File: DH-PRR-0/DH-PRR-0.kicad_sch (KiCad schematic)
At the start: 0 parts

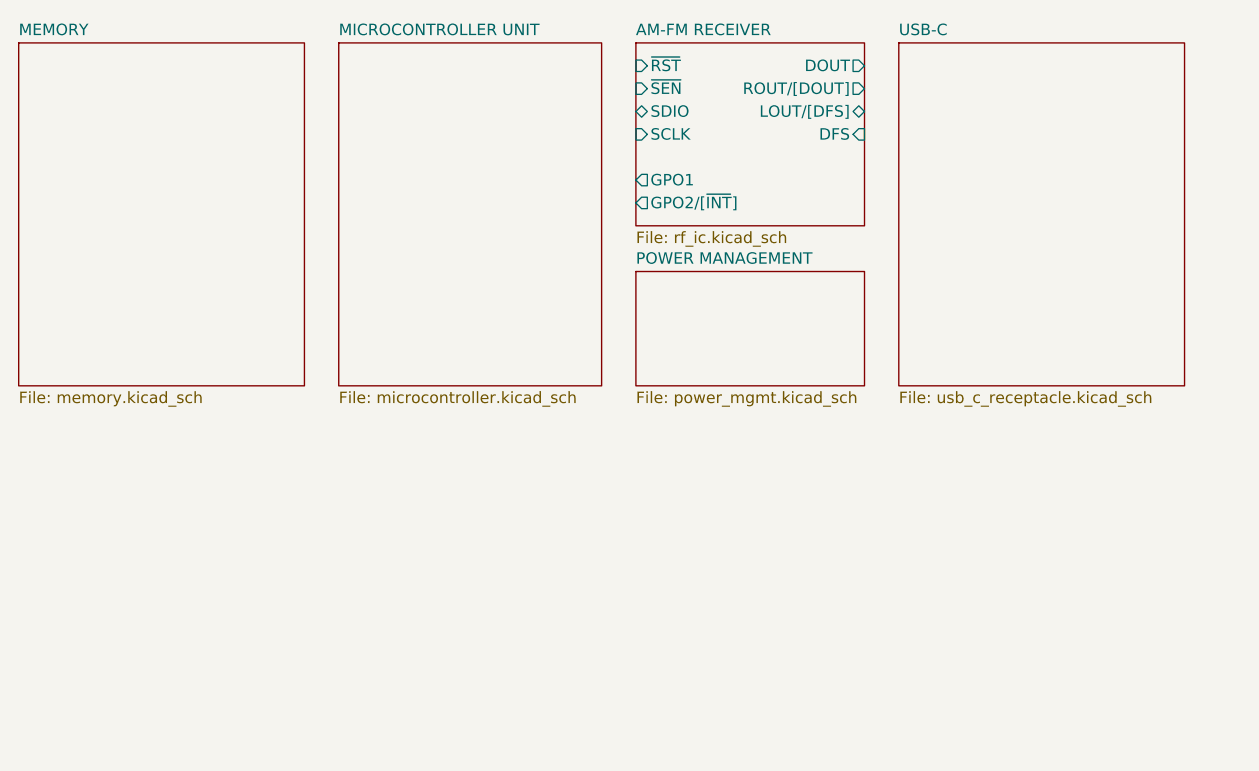
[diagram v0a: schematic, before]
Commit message: i dont remember
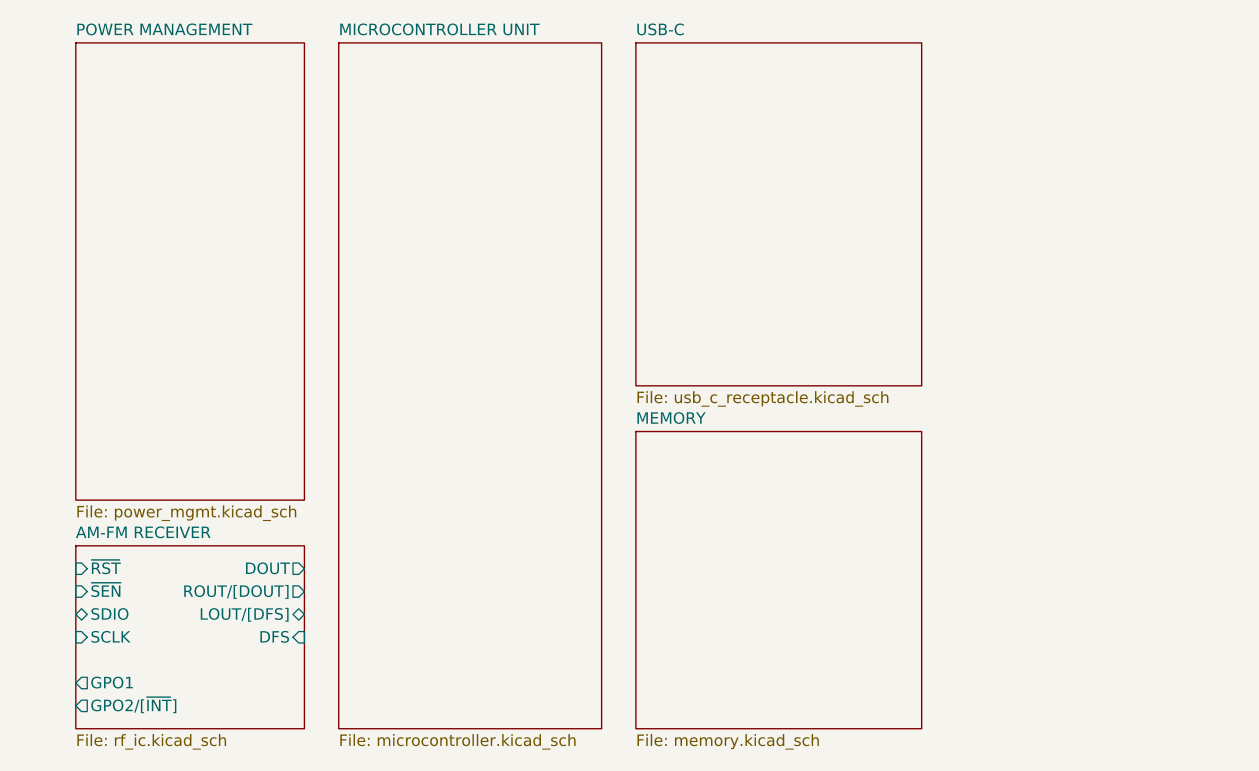
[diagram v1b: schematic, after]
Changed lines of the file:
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@@
 	(sheet
 		(at 60.96 25.4)
-		(size 29.21 38.1)
+		(size 29.21 76.2)
 		(exclude_from_sim no)
 		(in_bom yes)
@@
 		)
 		(property "Sheetfile" "microcontroller.kicad_sch"
-			(at 60.96 64.0846 0)
+			(at 60.96 102.1846 0)
 			(show_name no)
 			(do_not_autoplace no)
@@
 	)
 	(sheet
-		(at 25.4 25.4)
-		(size 31.75 38.1)
+		(at 93.98 68.58)
+		(size 31.75 33.02)
 		(exclude_from_sim no)
 		(in_bom yes)
@@
 		)
 		(property "Sheetname" "MEMORY"
-			(at 25.4 24.6884 0)
+			(at 93.98 67.8684 0)
 			(show_name no)
 			(do_not_autoplace no)
@@
 		)
 		(property "Sheetfile" "memory.kicad_sch"
-			(at 25.4 64.0846 0)
+			(at 93.98 102.1846 0)
 			(show_name no)
 			(do_not_autoplace no)
@@
 	)
 	(sheet
-		(at 93.98 25.4)
+		(at 31.75 81.28)
 		(size 25.4 20.32)
 		(exclude_from_sim no)
@@
 		)
 		(property "Sheetname" "AM-FM RECEIVER"
-			(at 93.98 24.6884 0)
+			(at 31.75 80.5684 0)
 			(show_name no)
 			(do_not_autoplace no)
@@
 		)
 		(property "Sheetfile" "rf_ic.kicad_sch"
-			(at 93.98 46.3046 0)
+			(at 31.75 102.1846 0)
 			(show_name no)
 			(do_not_autoplace no)
@@
 		)
 		(pin "DFS" input
-			(at 119.38 35.56 0)
+			(at 57.15 91.44 0)
 			(effects
 				(font
@@
 		)
 		(pin "DOUT" output
-			(at 119.38 27.94 0)
+			(at 57.15 83.82 0)
 			(effects
 				(font
@@
 		)
 		(pin "GPO1" output
-			(at 93.98 40.64 180)
+			(at 31.75 96.52 180)
 			(effects
 				(font
@@
 		)
 		(pin "GPO2/[~{INT}]" output
-			(at 93.98 43.18 180)
+			(at 31.75 99.06 180)
 			(effects
 				(font
@@
 		)
 		(pin "LOUT/[DFS]" bidirectional
-			(at 119.38 33.02 0)
+			(at 57.15 88.9 0)
 			(effects
 				(font
@@
 		)
 		(pin "ROUT/[DOUT]" output
-			(at 119.38 30.48 0)
+			(at 57.15 86.36 0)
 			(effects
 				(font
@@
 		)
 		(pin "SCLK" input
-			(at 93.98 35.56 180)
+			(at 31.75 91.44 180)
 			(effects
 				(font
@@
 		)
 		(pin "SDIO" bidirectional
-			(at 93.98 33.02 180)
+			(at 31.75 88.9 180)
 			(effects
 				(font
@@
 		)
 		(pin "~{RST}" input
-			(at 93.98 27.94 180)
+			(at 31.75 83.82 180)
 			(effects
 				(font
@@
 		)
 		(pin "~{SEN}" input
-			(at 93.98 30.48 180)
+			(at 31.75 86.36 180)
 			(effects
 				(font
@@
 	)
 	(sheet
-		(at 93.98 50.8)
-		(size 25.4 12.7)
+		(at 31.75 25.4)
+		(size 25.4 50.8)
 		(exclude_from_sim no)
 		(in_bom yes)
@@
 		)
 		(property "Sheetname" "POWER MANAGEMENT"
-			(at 93.98 50.0884 0)
+			(at 31.75 24.6884 0)
 			(show_name no)
 			(do_not_autoplace no)
@@
 		)
 		(property "Sheetfile" "power_mgmt.kicad_sch"
-			(at 93.98 64.0846 0)
+			(at 31.75 76.7846 0)
 			(show_name no)
 			(do_not_autoplace no)
@@
 	)
 	(sheet
-		(at 123.19 25.4)
+		(at 93.98 25.4)
 		(size 31.75 38.1)
 		(exclude_from_sim no)
@@
 		)
 		(property "Sheetname" "USB-C"
-			(at 123.19 24.6884 0)
+			(at 93.98 24.6884 0)
 			(show_name no)
 			(do_not_autoplace no)
@@
 		)
 		(property "Sheetfile" "usb_c_receptacle.kicad_sch"
-			(at 123.19 64.0846 0)
-			(show_name no)
-			(do_not_autoplace no)
+			(at 93.98 64.0846 0)
+			(show_name no)
+			(do_not_autoplace no)
